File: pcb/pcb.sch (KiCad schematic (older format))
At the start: 17 parts, among them J1 Barrel_Jack, J2 Barrel_Jack, J3 Screw_Terminal_01x03, J4 Screw_Terminal_01x02, J5 Conn_02x05_Odd_Even, J6 Conn_01x06_Male, SW1 SW_SPDT, U1 CPC5001G

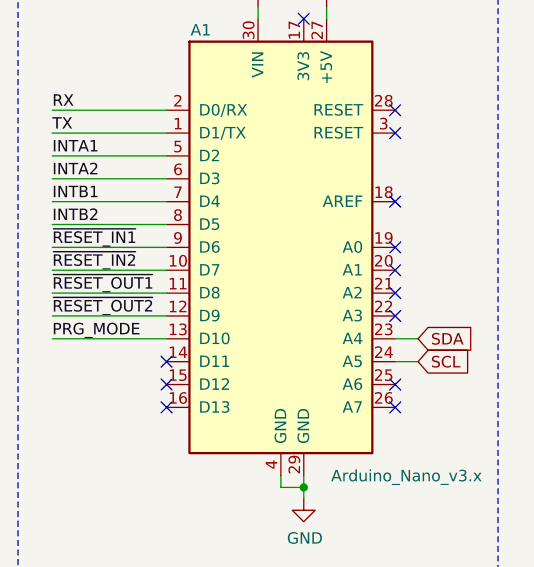
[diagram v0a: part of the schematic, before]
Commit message: update
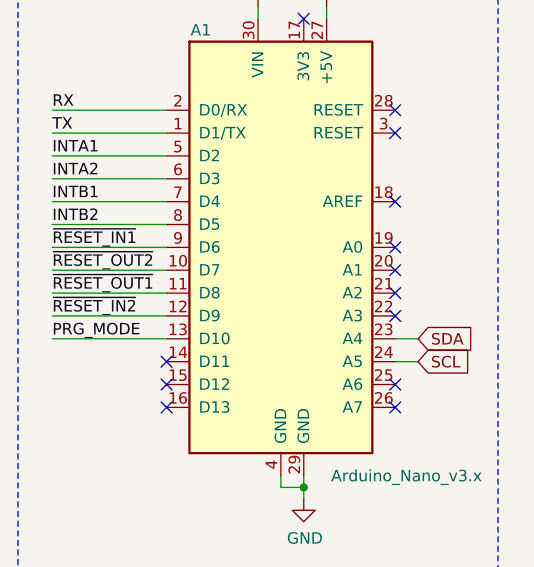
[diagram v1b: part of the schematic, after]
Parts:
- H1, H2, H3, H4: footprint MountingHole:MountingHole_4.3mm_M4 -> MountingHole:MountingHole_3.2mm_M3
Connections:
- net ~RESET_IN2: now also A1.12 (D9); no longer A1.10 (D7)
- net ~RESET_OUT2: now also A1.10 (D7); no longer A1.12 (D9)
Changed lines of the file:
@@
 F 0 "H1" H 5000 1296 50  0000 L CNN
 F 1 "MountingHole" H 5000 1205 50  0000 L CNN
-F 2 "MountingHole:MountingHole_4.3mm_M4" H 4900 1250 50  0001 C CNN
+F 2 "MountingHole:MountingHole_3.2mm_M3" H 4900 1250 50  0001 C CNN
 F 3 "~" H 4900 1250 50  0001 C CNN
 	1    4900 1250
@@
 F 0 "H2" H 5000 1546 50  0000 L CNN
 F 1 "MountingHole" H 5000 1455 50  0000 L CNN
-F 2 "MountingHole:MountingHole_4.3mm_M4" H 4900 1500 50  0001 C CNN
+F 2 "MountingHole:MountingHole_3.2mm_M3" H 4900 1500 50  0001 C CNN
 F 3 "~" H 4900 1500 50  0001 C CNN
 	1    4900 1500
@@
 F 0 "H3" H 5000 1796 50  0000 L CNN
 F 1 "MountingHole" H 5000 1705 50  0000 L CNN
-F 2 "MountingHole:MountingHole_4.3mm_M4" H 4900 1750 50  0001 C CNN
+F 2 "MountingHole:MountingHole_3.2mm_M3" H 4900 1750 50  0001 C CNN
 F 3 "~" H 4900 1750 50  0001 C CNN
 	1    4900 1750
@@
 F 0 "H4" H 5000 2046 50  0000 L CNN
 F 1 "MountingHole" H 5000 1955 50  0000 L CNN
-F 2 "MountingHole:MountingHole_4.3mm_M4" H 4900 2000 50  0001 C CNN
+F 2 "MountingHole:MountingHole_3.2mm_M3" H 4900 2000 50  0001 C CNN
 F 3 "~" H 4900 2000 50  0001 C CNN
 	1    4900 2000
@@
 Text Label 950  3850 0    50   ~ 0
 ~RESET_IN1
-Text Label 950  3950 0    50   ~ 0
+Text Label 950  4150 0    50   ~ 0
 ~RESET_IN2
 Text Label 950  4050 0    50   ~ 0
 ~RESET_OUT1
-Text Label 950  4150 0    50   ~ 0
+Text Label 950  3950 0    50   ~ 0
 ~RESET_OUT2
 Wire Wire Line

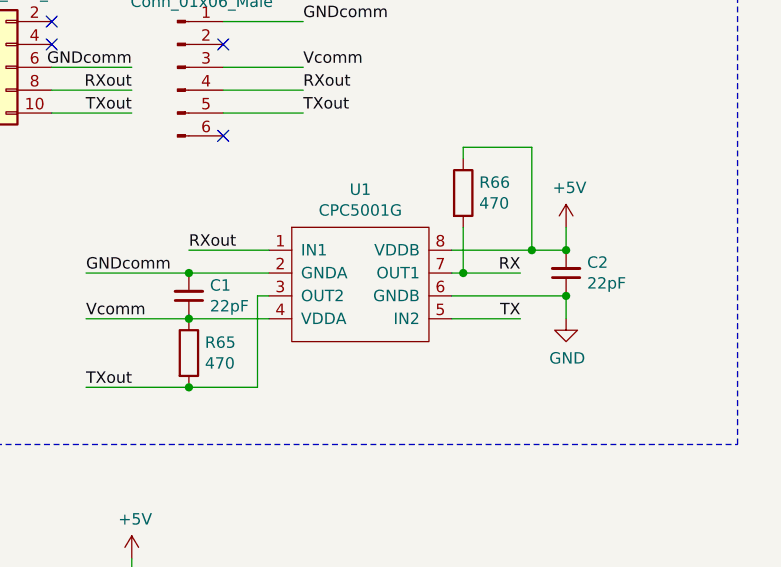
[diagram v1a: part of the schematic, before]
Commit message: Update
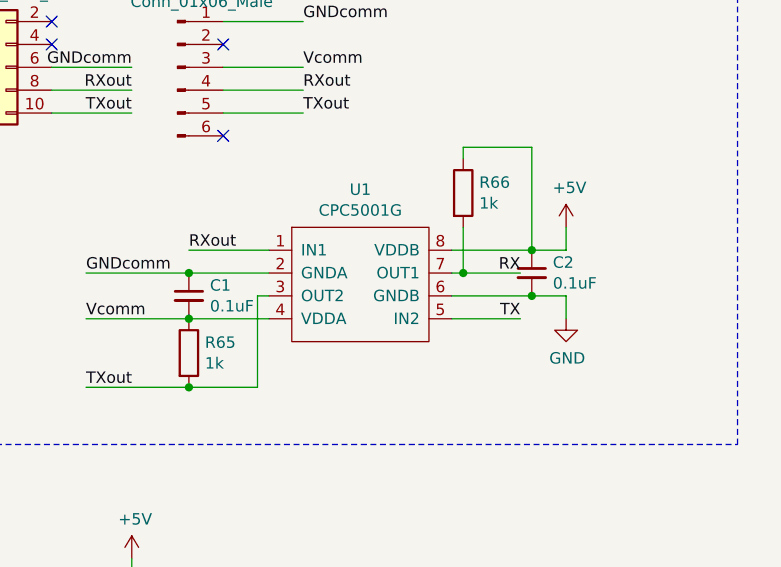
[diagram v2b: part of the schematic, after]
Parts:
- C1, C2: value 22pF -> 0.1uF
- H1, H2, H3, H4: footprint MountingHole:MountingHole_3.2mm_M3 -> MountingHole:MountingHole_4.3mm_M4
- R65, R66: value 470 -> 1k
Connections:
- net +5V: now also C2.1; no longer C2.2
- net GND: now also C2.2; no longer C2.1
- net GNDcomm: now also C1.1; no longer C1.2
- net Vcomm: now also C1.2; no longer C1.1
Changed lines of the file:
@@
 F 0 "H1" H 5000 1296 50  0000 L CNN
 F 1 "MountingHole" H 5000 1205 50  0000 L CNN
-F 2 "MountingHole:MountingHole_3.2mm_M3" H 4900 1250 50  0001 C CNN
+F 2 "MountingHole:MountingHole_4.3mm_M4" H 4900 1250 50  0001 C CNN
 F 3 "~" H 4900 1250 50  0001 C CNN
 	1    4900 1250
@@
 F 0 "H2" H 5000 1546 50  0000 L CNN
 F 1 "MountingHole" H 5000 1455 50  0000 L CNN
-F 2 "MountingHole:MountingHole_3.2mm_M3" H 4900 1500 50  0001 C CNN
+F 2 "MountingHole:MountingHole_4.3mm_M4" H 4900 1500 50  0001 C CNN
 F 3 "~" H 4900 1500 50  0001 C CNN
 	1    4900 1500
@@
 F 0 "H3" H 5000 1796 50  0000 L CNN
 F 1 "MountingHole" H 5000 1705 50  0000 L CNN
-F 2 "MountingHole:MountingHole_3.2mm_M3" H 4900 1750 50  0001 C CNN
+F 2 "MountingHole:MountingHole_4.3mm_M4" H 4900 1750 50  0001 C CNN
 F 3 "~" H 4900 1750 50  0001 C CNN
 	1    4900 1750
@@
 F 0 "H4" H 5000 2046 50  0000 L CNN
 F 1 "MountingHole" H 5000 1955 50  0000 L CNN
-F 2 "MountingHole:MountingHole_3.2mm_M3" H 4900 2000 50  0001 C CNN
+F 2 "MountingHole:MountingHole_4.3mm_M4" H 4900 2000 50  0001 C CNN
 F 3 "~" H 4900 2000 50  0001 C CNN
 	1    4900 2000
@@
 	1    0    0    -1
 $EndComp
-$Comp
-L Device:C_Small C1
-U 1 1 5C2A0087
-P 7650 2450
-F 0 "C1" H 7558 2404 50  0000 R CNN
-F 1 "22pF" H 7558 2495 50  0000 R CNN
-F 2 "Capacitor_THT:C_Disc_D5.0mm_W2.5mm_P2.50mm" H 7650 2450 50  0001 C CNN
-F 3 "~" H 7650 2450 50  0001 C CNN
-	1    7650 2450
-	-1   0    0    1
-$EndComp
 Wire Wire Line
 	8000 2550 7650 2550
 Wire Wire Line
-	8000 2350 7650 2350
-$Comp
-L Device:C_Small C2
-U 1 1 5C2A4A63
-P 9300 2350
-F 0 "C2" H 9208 2304 50  0000 R CNN
-F 1 "22pF" H 9208 2395 50  0000 R CNN
-F 2 "Capacitor_THT:C_Disc_D5.0mm_W2.5mm_P2.50mm" H 9300 2350 50  0001 C CNN
-F 3 "~" H 9300 2350 50  0001 C CNN
-	1    9300 2350
-	-1   0    0    1
-$EndComp
-Wire Wire Line
 	9300 2250 9150 2250
 Wire Wire Line
-	8800 2450 9300 2450
+	8800 2450 9150 2450
 Text Label 7200 2350 0    50   ~ 0
 GNDcomm
@@
 Vcomm
 Connection ~ 7650 2550
-Connection ~ 7650 2350
-Wire Wire Line
-	7200 2350 7650 2350
 Wire Wire Line
 	7200 2550 7650 2550
 Wire Wire Line
 	9300 2250 9300 2150
-Connection ~ 9300 2250
 $Comp
 L power:+5V #PWR0103
@@
 Wire Wire Line
 	9300 2450 9300 2550
-Connection ~ 9300 2450
 Wire Wire Line
 	8800 2350 8850 2350
@@
 P 8850 2000
 F 0 "R66" H 8920 2046 50  0000 L CNN
-F 1 "470" H 8920 1955 50  0000 L CNN
+F 1 "1k" H 8920 1955 50  0000 L CNN
 F 2 "Resistor_THT:R_Axial_DIN0207_L6.3mm_D2.5mm_P7.62mm_Horizontal" V 8780 2000 50  0001 C CNN
 F 3 "~" H 8850 2000 50  0001 C CNN
@@
 P 7650 2700
 F 0 "R65" H 7720 2746 50  0000 L CNN
-F 1 "470" H 7720 2655 50  0000 L CNN
+F 1 "1k" H 7720 2655 50  0000 L CNN
 F 2 "Resistor_THT:R_Axial_DIN0207_L6.3mm_D2.5mm_P7.62mm_Horizontal" V 7580 2700 50  0001 C CNN
 F 3 "~" H 7650 2700 50  0001 C CNN
@@
 Text Label 7200 2850 0    50   ~ 0
 TXout
+Wire Wire Line
+	7200 2350 7650 2350
+$Comp
+L Device:C_Small C1
+U 1 1 5C2EE7BD
+P 7650 2450
+F 0 "C1" H 7742 2496 50  0000 L CNN
+F 1 "0.1uF" H 7742 2405 50  0000 L CNN
+F 2 "Capacitor_THT:C_Disc_D5.0mm_W2.5mm_P2.50mm" H 7650 2450 50  0001 C CNN
+F 3 "~" H 7650 2450 50  0001 C CNN
+	1    7650 2450
+	1    0    0    -1
+$EndComp
+Connection ~ 7650 2350
+Wire Wire Line
+	7650 2350 8000 2350
+$Comp
+L Device:C_Small C2
+U 1 1 5C2EE82F
+P 9150 2350
+F 0 "C2" H 9242 2396 50  0000 L CNN
+F 1 "0.1uF" H 9242 2305 50  0000 L CNN
+F 2 "Capacitor_THT:C_Disc_D5.0mm_W2.5mm_P2.50mm" H 9150 2350 50  0001 C CNN
+F 3 "~" H 9150 2350 50  0001 C CNN
+	1    9150 2350
+	1    0    0    -1
+$EndComp
+Connection ~ 9150 2450
+Wire Wire Line
+	9150 2450 9300 2450
 $EndSCHEMATC
